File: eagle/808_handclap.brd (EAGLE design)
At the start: 100 x 80 mm, 82 parts, among them IC1 LM339N, IC2 TL071P, IC3 TL071P, Q1 2N3906, Q2 2N3904, Q3 2N3906, Q4 2N3906, Q5 2N3904, Q6 2N3904, Q7 2N3904, U1 POWER, U22 BA6110SIL

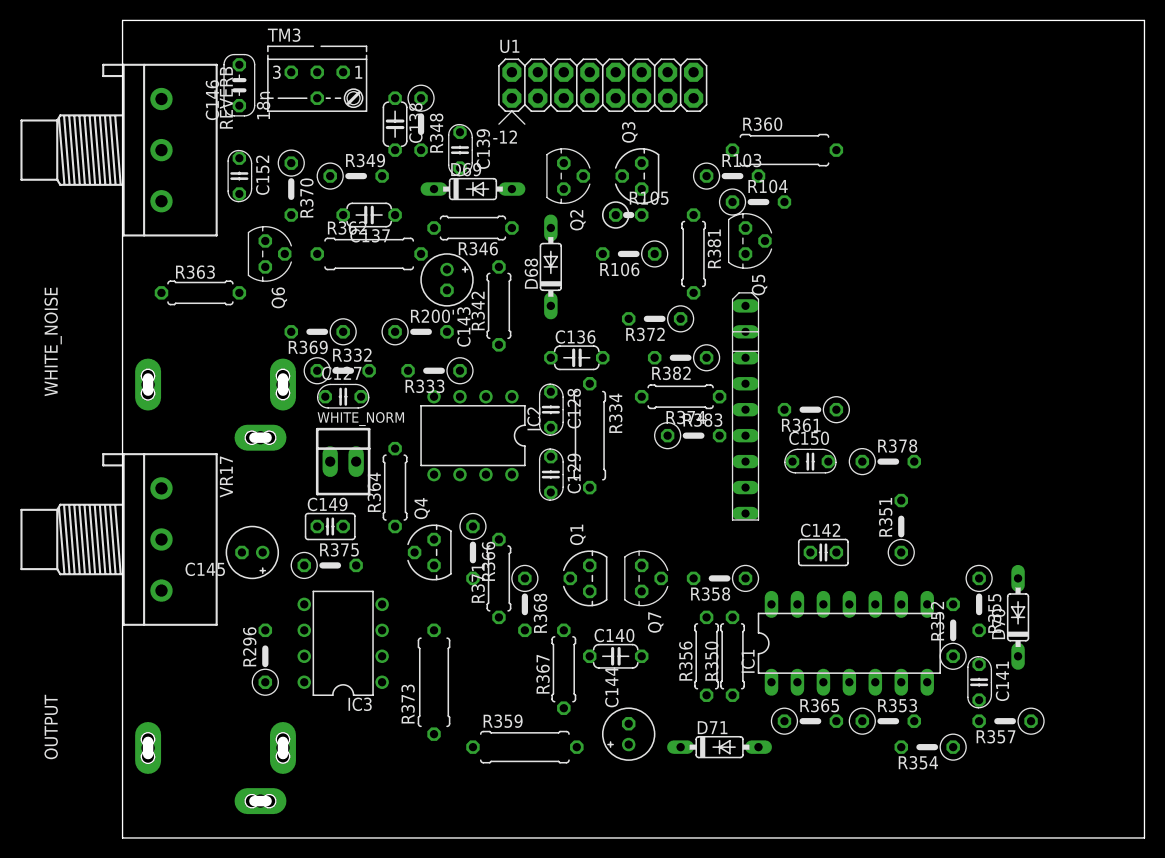
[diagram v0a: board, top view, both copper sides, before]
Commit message: manual mode
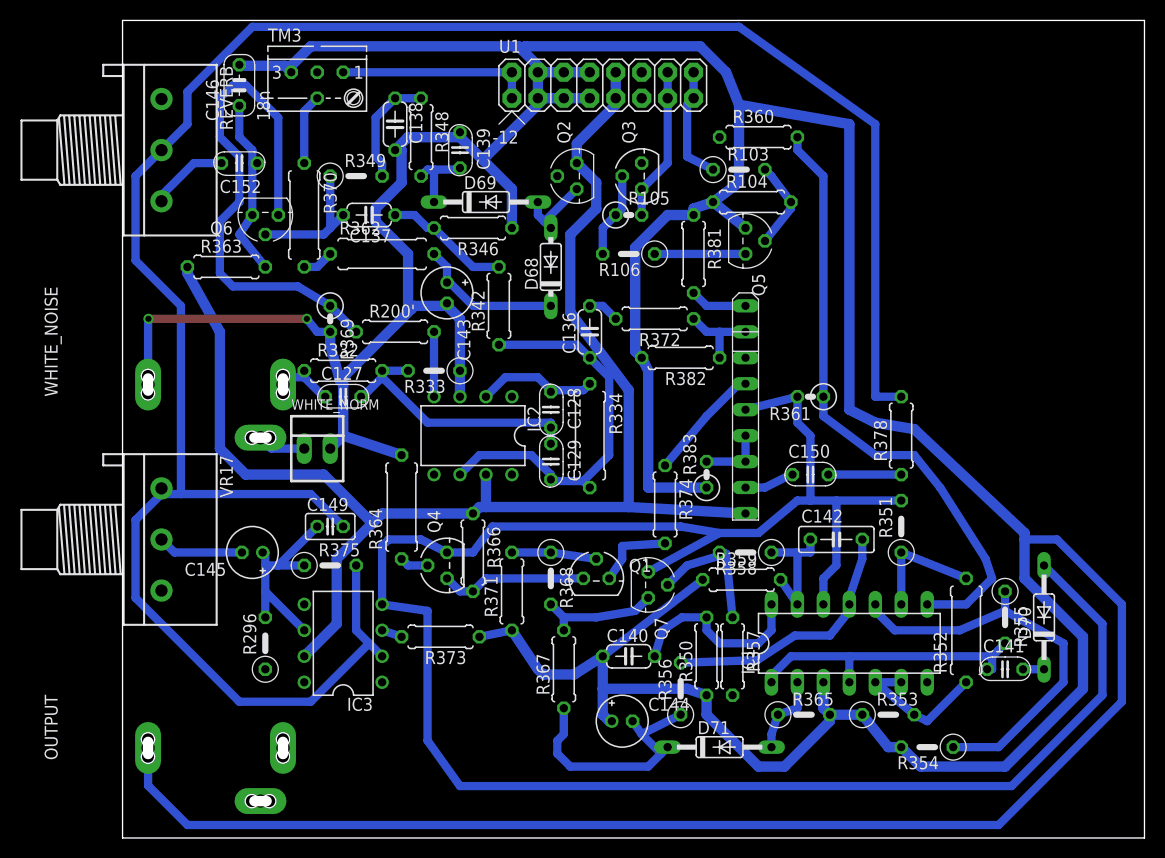
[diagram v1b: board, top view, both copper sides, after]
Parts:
- C142: device TR808clone:C025-025X050 -> TR808clone:C050-025X075
- D69, D70, D71: value 1N4148DO35-7 -> 1N4148DO35-10; device TR808clone:DO35-7 -> TR808clone:DO35-10
- R104, R200', R332, R348, R357, R366, R372, R378, R382: device TR808clone:0207/5V -> TR808clone:0207/7
- R352, R370: device TR808clone:0207/5V -> TR808clone:0309/10
- R356: device TR808clone:0207/7 -> TR808clone:0207/5V
- R359, R360, R373: device TR808clone:0309/10 -> TR808clone:0207/7
- R361, R369, R383: device TR808clone:0207/5V -> TR808clone:0207/2V
- R364: device TR808clone:0207/7 -> TR808clone:0309/10
- moved R357 27.4 mm to (59.7, 17.8), turned to 270 degrees
- moved R359 26.8 mm to (60.6, 25.3)
- moved R374 10.7 mm to (53.1, 32.6), turned to 270 degrees
- moved R373 4.49 mm to (31.1, 19.7), turned to 180 degrees
- moved R356 4.07 mm to (54.6, 14.6)
- moved R383 4.02 mm to (57.1, 35.6), turned to 90 degrees
- moved Q6 3.81 mm to (14.0, 61.0), turned to 180 degrees
- moved R358 3.59 mm to (61.0, 27.9)
- moved R363 3.59 mm to (10.2, 55.9)
- moved R368 3.59 mm to (41.9, 25.4)
- moved C141 2.84 mm to (86.4, 16.5), turned to 0 degrees
- moved R355 2.84 mm to (86.4, 21.6)
- moved WHITE_NORM 2.84 mm to (19.1, 38.1)
- moved R370 2.84 mm to (17.8, 61.0)
- moved C136 2.84 mm to (45.7, 49.5), turned to 90 degrees
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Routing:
- net GND: track 0.00 -> 537.8 mm, vias 0 -> 2
- net -12V: track 0.00 -> 224.4 mm
- net N$92: track 0.00 -> 215.8 mm
- net +12V: track 0.00 -> 140.6 mm
- net N$74: track 0.00 -> 60.3 mm
- net N$42: track 0.00 -> 51.2 mm
- net N$73: track 0.00 -> 40.2 mm
- net N$10: track 0.00 -> 38.5 mm
- net N$68: track 0.00 -> 29.1 mm
- net N$52: track 0.00 -> 26.4 mm
- net N$72: track 0.00 -> 25.6 mm
- net N$65: track 0.00 -> 25.3 mm
- net N$97: track 0.00 -> 21.2 mm
- net N$77: track 0.00 -> 18.6 mm
- net N$46: track 0.00 -> 18.1 mm
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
